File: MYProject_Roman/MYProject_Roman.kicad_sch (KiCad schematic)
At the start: 74 parts, among them Q1 HC-49SMD-XTAL_MD

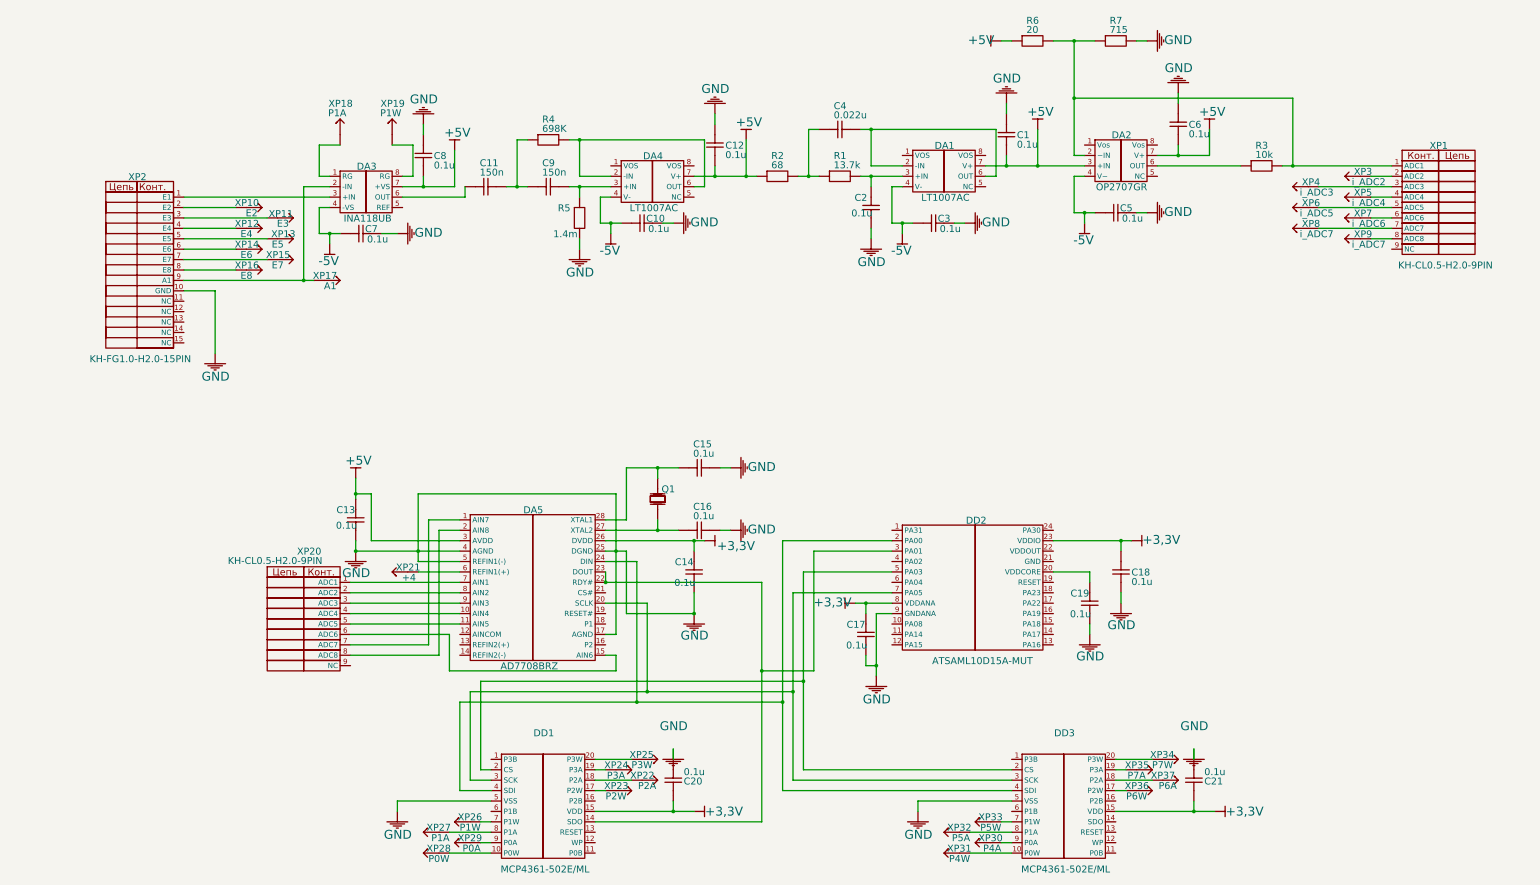
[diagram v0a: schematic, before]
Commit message: Добавлена копия проекта
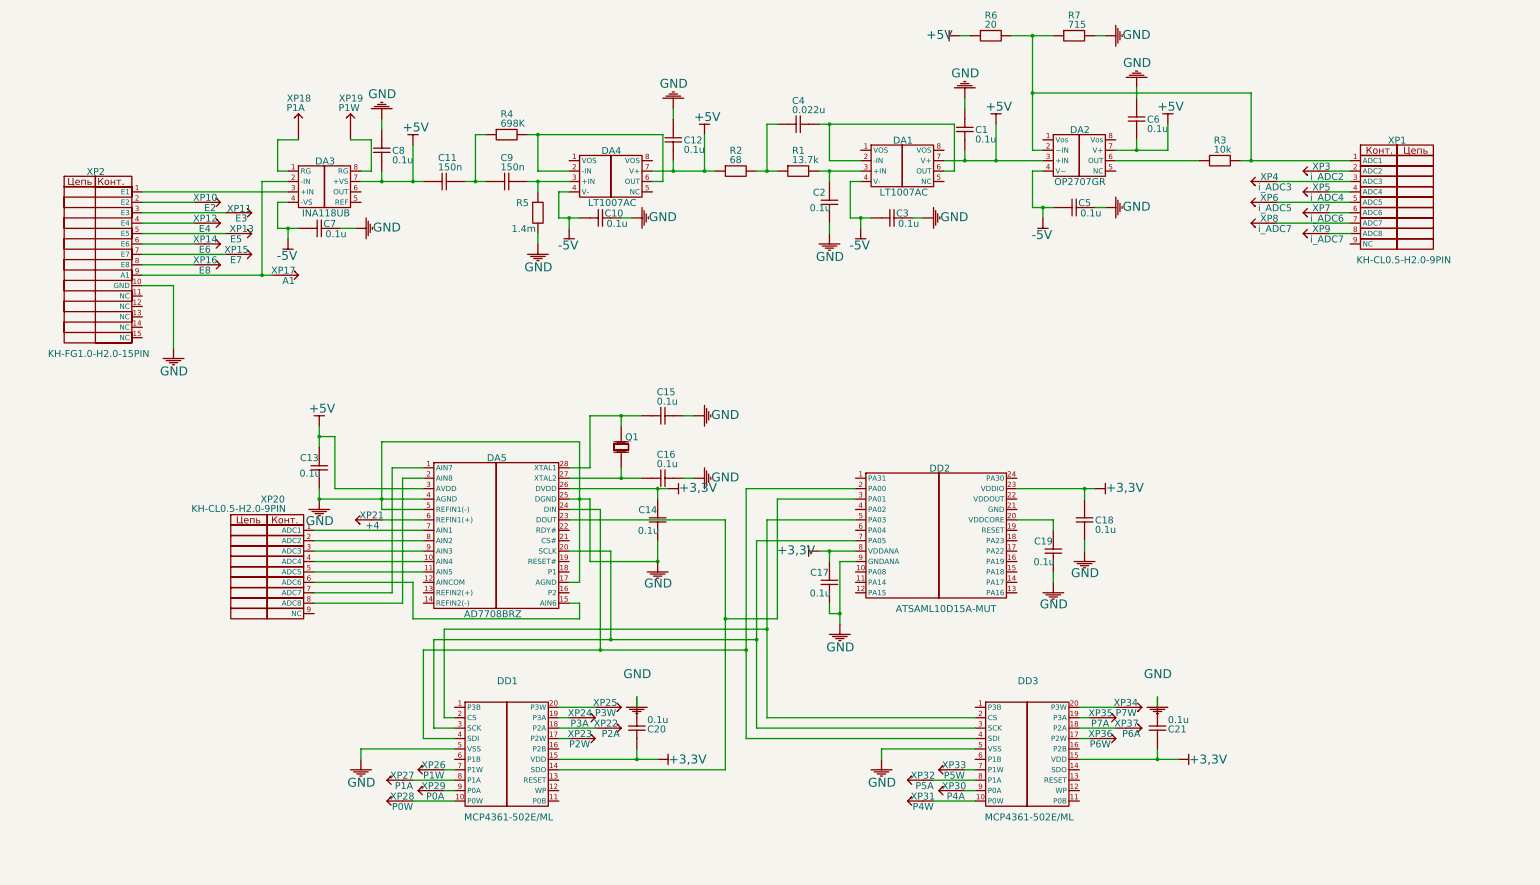
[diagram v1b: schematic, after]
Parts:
- removed XP1: KH-CL0.5-H2.0-9PIN, symbol KH-CL0.5-H2.0-9PIN
- added XP1: KH-CL0.5-H2.0-9PIN, symbol KH-CL0.5-H2.0-9PIN
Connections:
- net +5V: now also C11.1
- net at DA5.23 (DOUT), DD1.14 (SDO), DD2.3 (PA01): no longer DA5.22 (RDY#)
- net at XP9.1: now also XP1.8 (ADC8)
- net at DA2.2 (−IN), R3.2, R6.2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: now also XP1.1 (ADC1)
- net at XP4.1: now also XP1.3 (ADC3)
- net at XP3.1: now also XP1.2 (ADC2)
- net at XP5.1: now also XP1.4 (ADC4)
- net at XP6.1: now also XP1.5 (ADC5)
- net at XP7.1: now also XP1.6 (ADC6)
- net at XP8.1: now also XP1.7 (ADC7)
- net at DA3.6 (OUT): no longer C11.1
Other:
- title: Регистратор ЭЭГ -> Тракт ЭЭГ регистратора
